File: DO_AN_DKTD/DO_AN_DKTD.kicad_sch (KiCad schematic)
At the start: 61 parts, among them J1 Conn_01x03, J2 Conn_01x02, J3 Conn_01x07, J4 Conn_01x04, J5 Conn_01x02, Q1 NPN, Q2 NPN, Q3 NPN, Q4 NPN, SW2 RotaryEncoder_Switch, U1 AMS1117, U2 74HC595, U3 MOC3020M, U4 PC817, U5 DevKitSTM32

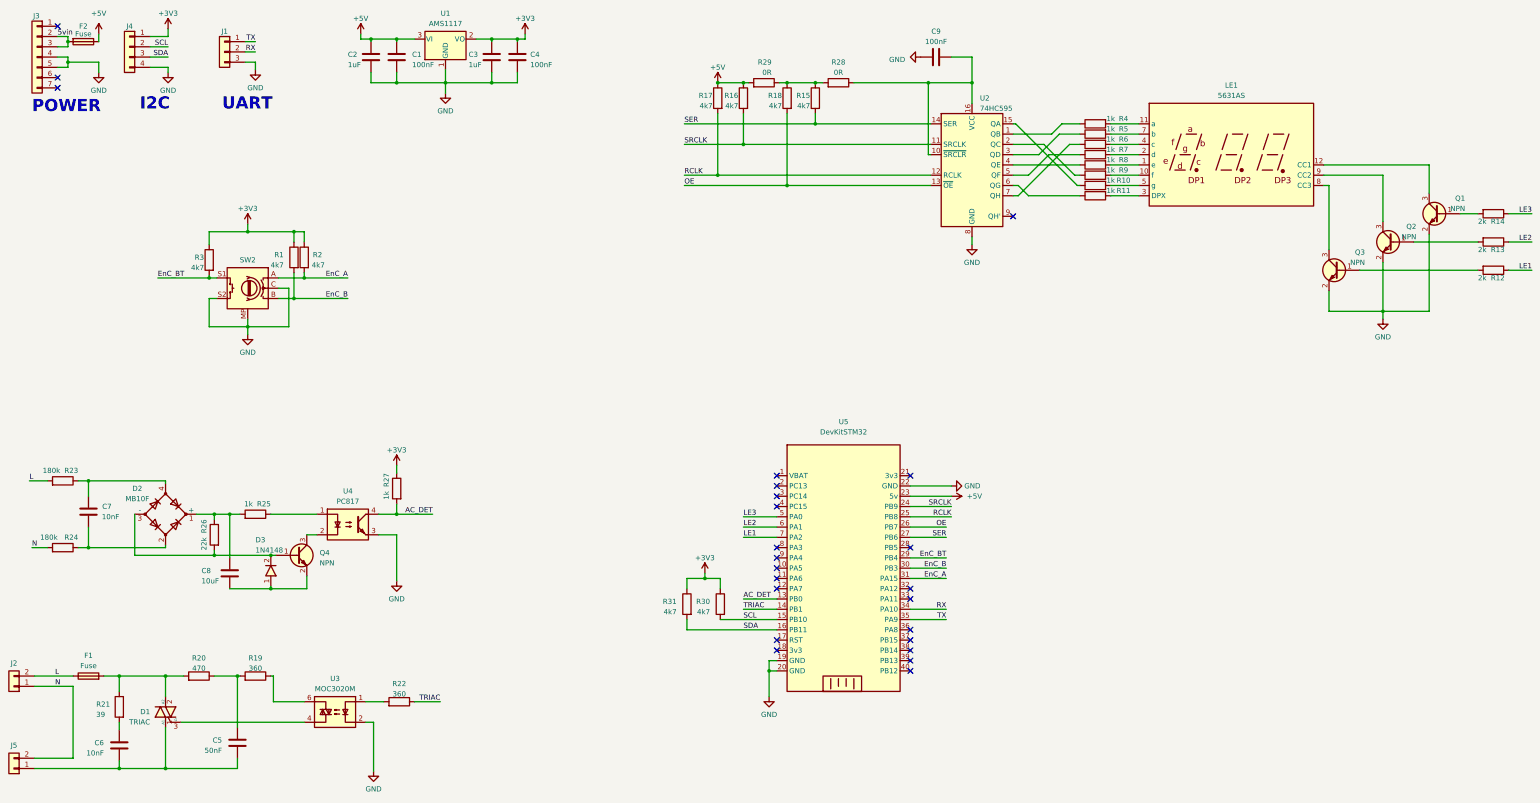
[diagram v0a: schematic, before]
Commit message: completed layout PCB Ver 1.0
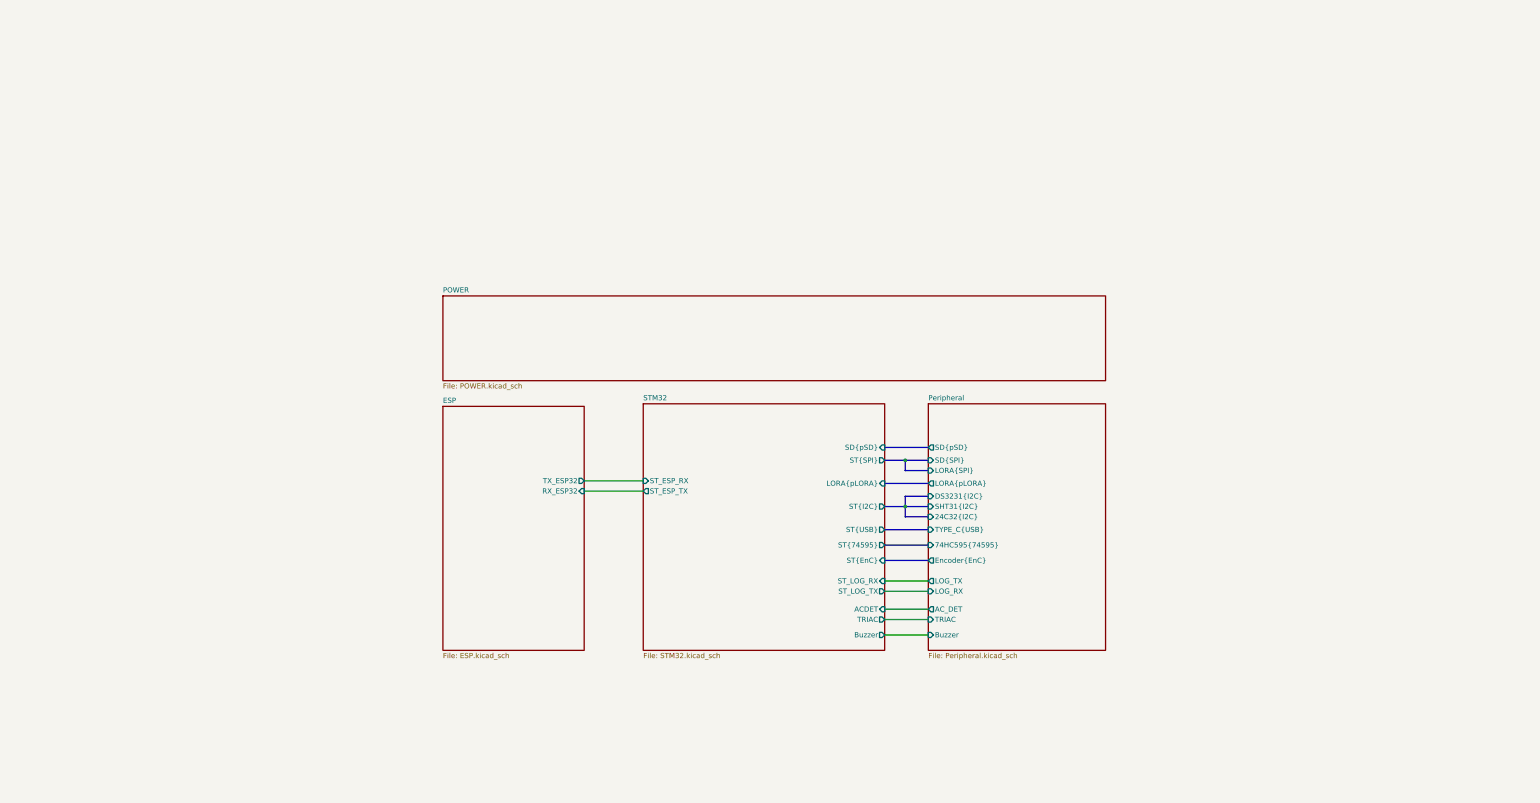
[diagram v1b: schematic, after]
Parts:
- removed C1, C4, C9: 100nF, IVS_FOOTPRINTS:C_0603, symbol Device:C
- removed C2, C3: 1uF, IVS_FOOTPRINTS:C_0603, symbol Device:C
- removed C5: 50nF, IVS_FOOTPRINTS:C_0603, symbol Device:C
- removed C6, C7: 10nF, IVS_FOOTPRINTS:C_0603, symbol Device:C
- removed C8: 10uF, IVS_FOOTPRINTS:C_0603, symbol Device:C
- removed D1: TRIAC, IVS_FOOTPRINTS:TO-220-3_Vertical, symbol IVS_SYMBOLS:Triac
- removed D2: MB10F, IVS_FOOTPRINTS:Bridge_MB10F-13, symbol Device:D_Bridge_+A-A
- removed D3: 1N4148, IVS_FOOTPRINTS:D_SOD323, symbol IVS_SYMBOLS:D_Diode
- removed F1: Fuse, IVS_FOOTPRINTS:Fuse_BLX-A-P22.4mm, symbol IVS_SYMBOLS:Fuse
- removed F2: Fuse, IVS_FOOTPRINTS:Fuse_1812_4532Metric, symbol IVS_SYMBOLS:Fuse
- removed J1: Conn_01x03, IVS_FOOTPRINTS:Conn_XH-P2.54mm-3P, symbol Connector_Generic:Conn_01x03
- removed J2, J5: Conn_01x02, IVS_FOOTPRINTS:KF128-5.0-2P, symbol Connector_Generic:Conn_01x02
- removed J3: Conn_01x07, IVS_FOOTPRINTS:Conn_XH-P2.54mm-7P, symbol Connector_Generic:Conn_01x07
- removed J4: Conn_01x04, IVS_FOOTPRINTS:Conn_XH-P2.54mm-4P, symbol Connector_Generic:Conn_01x04
- removed LE1: 5631AS, IVS_FOOTPRINTS:7Segment_4led_CC_38x19, symbol IVS_SYMBOLS:7seg_5631AS
- removed Q1, Q2, Q3, Q4: NPN, IVS_FOOTPRINTS:SOT23-3, symbol IVS_SYMBOLS:NPN
- removed R1, R15, R16, R17, R18, R2, R3, R30, R31: 4k7, IVS_FOOTPRINTS:R0603, symbol Device:R
- removed R10, R11, R25, R27, R4, R5, R6, R7, R8, R9: 1k, IVS_FOOTPRINTS:R0603, symbol Device:R
- removed R12, R13, R14: 2k, IVS_FOOTPRINTS:R0603, symbol Device:R
- removed R19: 360, IVS_FOOTPRINTS:R0805, symbol Device:R
- removed R20: 470, IVS_FOOTPRINTS:R0603, symbol Device:R
- removed R21: 39, IVS_FOOTPRINTS:R0603, symbol Device:R
- removed R22: 360, IVS_FOOTPRINTS:R0603, symbol Device:R
- removed R23, R24: 180k, IVS_FOOTPRINTS:R0603, symbol Device:R
- removed R26: 22k, IVS_FOOTPRINTS:R0603, symbol Device:R
- removed R28, R29: 0R, IVS_FOOTPRINTS:R0805, symbol Device:R
- removed SW2: RotaryEncoder_Switch, IVS_FOOTPRINTS:RotaryEncoder_Alps_EC11E-Switch_Vertical_H20mm, symbol IVS_SYMBOLS:RotaryEncoder_Switch
- removed U1: AMS1117, IVS_FOOTPRINTS:SOT233, symbol IVS_SYMBOLS:AMS1117
- removed U2: 74HC595, IVS_FOOTPRINTS:SOIC-16W_5.3x10.2mm_P1.27mm, symbol 74xx:74HC595
- removed U3: MOC3020M, IVS_FOOTPRINTS:DIL06-E, symbol Relay_SolidState:MOC3020M
- removed U4: PC817, IVS_FOOTPRINTS:OPTO_SOT254P975X400-4N, symbol Isolator:EL817
- removed U5: DevKitSTM32, IVS_FOOTPRINTS:DevKitSTM32, symbol IVS_SYMBOLS:DevKitSTM32
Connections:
- no-connect marks 24 -> 0
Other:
- added sheet ESP (ESP.kicad_sch)
- added sheet POWER (POWER.kicad_sch)
- added sheet Peripheral (Peripheral.kicad_sch)
- added sheet STM32 (STM32.kicad_sch)
- note removed: "I2C"
- note removed: "POWER"
- note removed: "UART"
